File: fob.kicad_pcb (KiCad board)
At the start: 2 copper layers, 53 x 53 mm, 9 parts, among them P1 SW DBG, P2 SOIC16-ZIF

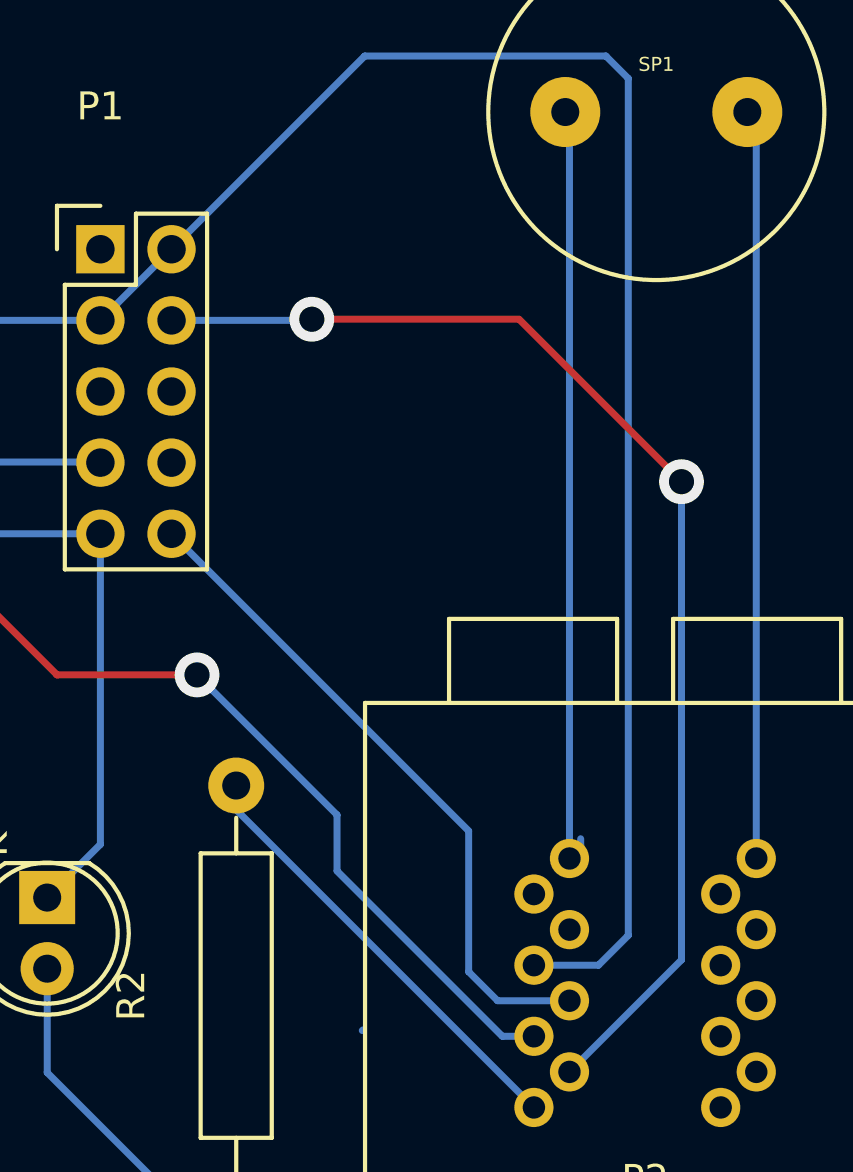
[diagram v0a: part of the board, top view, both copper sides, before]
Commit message: got version 1.1 ready to cut
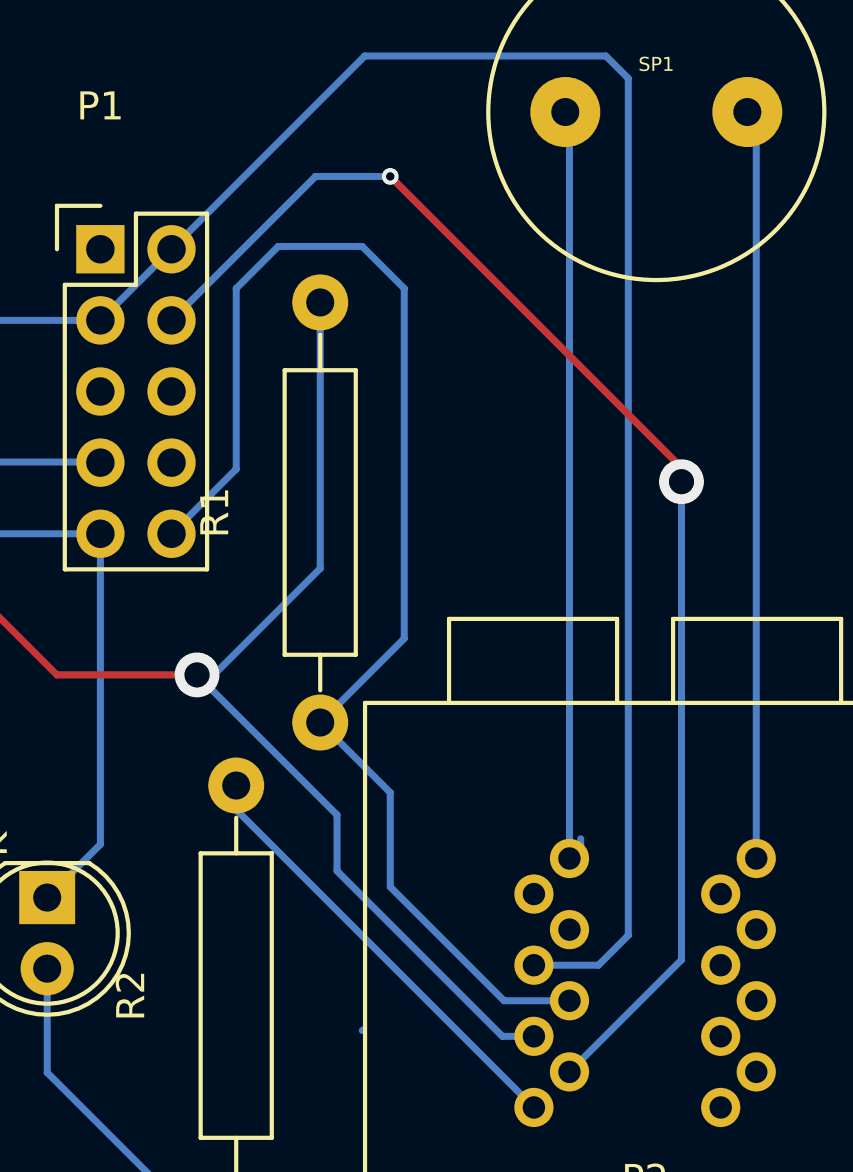
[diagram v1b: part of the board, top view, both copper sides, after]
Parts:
- added R1: 10K, Resistors_ThroughHole:Resistor_Horizontal_RM15mm, F.Cu at (128.5, 96.5)
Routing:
- net VDD: track 24.1 -> 48.7 mm
- net Net-(P1-Pad7): track 37.4 -> 52.9 mm
- net Net-(P1-Pad4): track 43.4 -> 47.9 mm
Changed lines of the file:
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@@
 (kicad_pcb (version 4) (host pcbnew "(2015-06-01 BZR 5694)-product")
   (general
-    (links 11)
+    (links 13)
     (no_connects 0)
-    (area 106.949999 74.949999 160.050001 128.050001)
+    (area 105.511474 74.8745 163.490046 128.97626)
     (thickness 1.6)
     (drawings 4)
-    (tracks 51)
+    (tracks 62)
     (zones 0)
-    (modules 9)
+    (modules 10)
     (nets 13)
   )
@@
     (title "Form Of Bee")
     (date "Wed 26 Aug 2015")
-    (rev 1.0b)
+    (rev 1.1)
     (company "Bart Massey")
     (comment 1 "Copyright 2015 Bart Massey")
@@
     (pad "" thru_hole circle (at 0 0) (size 3.5 3.5) (drill 3.5) (layers *.Cu *.Mask F.SilkS))
   )
+  (module Resistors_ThroughHole:Resistor_Horizontal_RM15mm (layer F.Cu)
+    (at 128.5 96.5 90)
+    (descr "Resistor, Axial, RM 15mm,")
+    (tags "Resistor, Axial, RM 15mm,")
+    (fp_text reference R1 (at 0 -3.74904 90) (layer F.SilkS)
+      (effects (font (size 1 1) (thickness 0.15)))
+    )
+    (fp_text value 10K (at 0 4.0005 90) (layer F.Fab)
+      (effects (font (size 1 1) (thickness 0.15)))
+    )
+    (fp_line (start -5.08 -1.27) (end -5.08 1.27) (layer F.SilkS) (width 0.15))
+    (fp_line (start -5.08 1.27) (end 5.08 1.27) (layer F.SilkS) (width 0.15))
+    (fp_line (start 5.08 1.27) (end 5.08 -1.27) (layer F.SilkS) (width 0.15))
+    (fp_line (start 5.08 -1.27) (end -5.08 -1.27) (layer F.SilkS) (width 0.15))
+    (fp_line (start 6.35 0) (end 5.08 0) (layer F.SilkS) (width 0.15))
+    (fp_line (start -6.35 0) (end -5.08 0) (layer F.SilkS) (width 0.15))
+    (pad 1 thru_hole circle (at -7.5 0 90) (size 1.99898 1.99898) (drill 1.00076) (layers *.Cu *.SilkS *.Mask)
+      (net 9 VDD))
+    (pad 2 thru_hole circle (at 7.5 0 90) (size 1.99898 1.99898) (drill 1.00076) (layers *.Cu *.SilkS *.Mask)
+      (net 7 "Net-(P1-Pad7)"))
+    (model Resistors_ThroughHole.3dshapes/Resistor_Horizontal_RM15mm.wrl
+      (at (xyz 0 0 0))
+      (scale (xyz 0.4 0.4 0.4))
+      (rotate (xyz 0 0 0))
+    )
+  )
   (gr_line (start 107 128) (end 107 75) (angle 90) (layer Edge.Cuts) (width 0.1))
   (gr_line (start 160 128) (end 107 128) (angle 90) (layer Edge.Cuts) (width 0.1))
@@
   (segment (start 118.75 116.5) (end 118.75 112.79) (width 0.25) (layer B.Cu) (net 2))
   (segment (start 123.5 121.25) (end 118.75 116.5) (width 0.25) (layer B.Cu) (net 2))
+  (segment (start 141.4 95.4) (end 141.4 94.9) (width 0.25) (layer F.Cu) (net 4))
+  (segment (start 137.4 116.475) (end 141.4 112.475) (width 0.25) (layer B.Cu) (net 4))
+  (via (at 141.4 95.4) (size 1.6) (drill 0.9) (layers F.Cu B.Cu) (net 4))
   (segment (start 141.4 112.475) (end 141.4 95.4) (width 0.25) (layer B.Cu) (net 4))
-  (via (at 141.4 95.4) (size 1.6) (drill 0.9) (layers F.Cu B.Cu) (net 4))
-  (segment (start 141.4 95.4) (end 135.6 89.6) (width 0.25) (layer F.Cu) (net 4))
-  (segment (start 135.6 89.6) (end 128.2 89.6) (width 0.25) (layer F.Cu) (net 4))
-  (via (at 128.2 89.6) (size 1.6) (drill 0.9) (layers F.Cu B.Cu) (net 4))
-  (segment (start 128.2 89.6) (end 128.16 89.64) (width 0.25) (layer B.Cu) (net 4))
-  (segment (start 128.16 89.64) (end 123.19 89.64) (width 0.25) (layer B.Cu) (net 4))
-  (segment (start 137.4 116.475) (end 141.4 112.475) (width 0.25) (layer B.Cu) (net 4))
+  (segment (start 128.33 84.5) (end 123.19 89.64) (width 0.25) (layer B.Cu) (net 4))
+  (segment (start 131 84.5) (end 128.33 84.5) (width 0.25) (layer B.Cu) (net 4))
+  (via (at 131 84.5) (size 0.6) (layers F.Cu B.Cu) (net 4))
+  (segment (start 141.4 94.9) (end 131 84.5) (width 0.25) (layer F.Cu) (net 4))
+  (segment (start 128.5 89) (end 128.5 98.5) (width 0.25) (layer B.Cu) (net 7))
+  (segment (start 124.7 102.3) (end 124.1 102.3) (width 0.25) (layer B.Cu) (net 7))
+  (segment (start 128.5 98.5) (end 124.7 102.3) (width 0.25) (layer B.Cu) (net 7))
   (segment (start 120.65 94.72) (end 120.53 94.72) (width 0.25) (layer B.Cu) (net 7))
   (segment (start 120.63 94.7) (end 120.65 94.72) (width 0.25) (layer B.Cu) (net 7))
@@
   (segment (start 135.005 115.205) (end 129.1 109.3) (width 0.25) (layer B.Cu) (net 7))
   (segment (start 120.63 94.7) (end 115.9 94.7) (width 0.25) (layer B.Cu) (net 7))
-  (segment (start 134.835 113.935) (end 133.8 112.9) (width 0.25) (layer B.Cu) (net 9))
-  (segment (start 133.8 112.9) (end 133.8 107.87) (width 0.25) (layer B.Cu) (net 9))
-  (segment (start 133.8 107.87) (end 123.19 97.26) (width 0.25) (layer B.Cu) (net 9))
-  (segment (start 137.4 113.935) (end 134.835 113.935) (width 0.25) (layer B.Cu) (net 9))
+  (segment (start 128.2 89.6) (end 128.16 89.64) (width 0.25) (layer B.Cu) (net 7))
+  (segment (start 128.5 104) (end 131.5 101) (width 0.25) (layer B.Cu) (net 9))
+  (segment (start 125.5 94.95) (end 123.19 97.26) (width 0.25) (layer B.Cu) (net 9))
+  (segment (start 125.5 88.5) (end 125.5 94.95) (width 0.25) (layer B.Cu) (net 9))
+  (segment (start 127 87) (end 125.5 88.5) (width 0.25) (layer B.Cu) (net 9))
+  (segment (start 130 87) (end 127 87) (width 0.25) (layer B.Cu) (net 9))
+  (segment (start 131.5 88.5) (end 130 87) (width 0.25) (layer B.Cu) (net 9))
+  (segment (start 131.5 101) (end 131.5 88.5) (width 0.25) (layer B.Cu) (net 9))
+  (segment (start 137.4 113.935) (end 135.065 113.935) (width 0.25) (layer B.Cu) (net 9))
+  (segment (start 131 106.5) (end 128.5 104) (width 0.25) (layer B.Cu) (net 9))
+  (segment (start 131 109.87) (end 131 106.5) (width 0.25) (layer B.Cu) (net 9))
+  (segment (start 135.065 113.935) (end 131 109.87) (width 0.25) (layer B.Cu) (net 9))
   (segment (start 137.8 108.365) (end 137.8 108.15) (width 0.25) (layer B.Cu) (net 10))
   (segment (start 137.8 108.365) (end 137.8 108.55) (width 0.25) (layer B.Cu) (net 10))
